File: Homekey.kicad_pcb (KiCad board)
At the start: 2 copper layers, 41.6 x 47.3 mm, 71 parts, among them J1 Hirose, J2 Screw_Terminal_01x02, J3 USB_C_Receptacle_USB2.0_16P, U1 ESP32-C3-WROOM-02, U2 PN5321A3HN_C1xx, U3 MAX17501AxTB, U4 TLV75533PDRV, Y1 27.12MHz

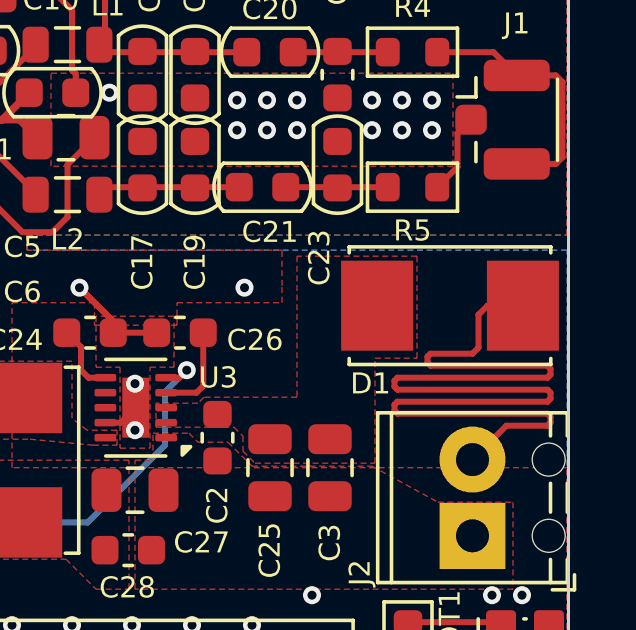
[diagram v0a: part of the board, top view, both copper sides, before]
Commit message: Adding gerbers + BOM
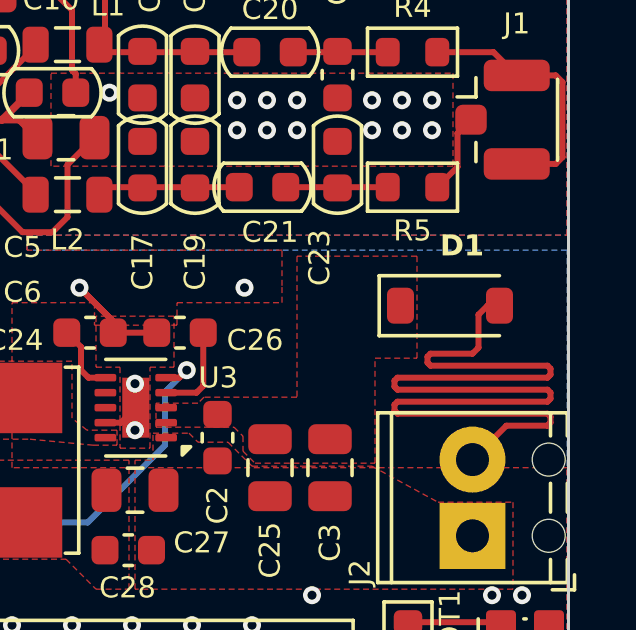
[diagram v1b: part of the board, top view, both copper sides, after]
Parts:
- D1: footprint Fuse:Fuseholder_Littelfuse_Nano2_157x -> Diode_SMD:D_SOD-123
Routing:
- net Net-(D1-A): track 34.2 -> 33.4 mm
